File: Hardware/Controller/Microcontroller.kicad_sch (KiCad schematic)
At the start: 26 parts, among them J201 TagConnect_SWD, SW201 SW_Push, SW202 SW_Push, U201 W25Q64JVXGIQ, U202 RP2040, Y201 12M

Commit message: Changes and fixes
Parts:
- Y201: footprint Crystal:Crystal_SMD_Abracon_ABM3B-4Pin_5.0x3.2mm -> Crystal:Crystal_SMD_2520-4Pin_2.5x2.0mm; mouser 815-ABM3B1210B1UT -> 520-120-10-36Q-AEST
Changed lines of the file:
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@@
-	)
-	(symbol
-		(lib_id "Device:Crystal_GND24")
-		(at 38.1 152.4 90)
-		(unit 1)
-		(exclude_from_sim no)
-		(in_bom yes)
-		(on_board yes)
-		(dnp no)
-		(property "Reference" "Y201"
-			(at 38.1 142.24 90)
-			(effects
-				(font
-					(size 1.27 1.27)
-				)
-			)
-		)
-		(property "Value" "12M"
-			(at 38.1 144.78 90)
-			(effects
-				(font
-					(size 1.27 1.27)
-				)
-			)
-		)
-		(property "Footprint" "Crystal:Crystal_SMD_Abracon_ABM3B-4Pin_5.0x3.2mm"
-			(at 38.1 152.4 0)
-			(effects
-				(font
-					(size 1.27 1.27)
-				)
-				(hide yes)
-			)
-		)
-		(property "Datasheet" "https://eu.mouser.com/datasheet/2/3/abm3b-1774998.pdf"
-			(at 38.1 152.4 0)
-			(effects
-				(font
-					(size 1.27 1.27)
-				)
-				(hide yes)
-			)
-		)
-		(property "Description" ""
-			(at 38.1 152.4 0)
-			(effects
-				(font
-					(size 1.27 1.27)
-				)
-				(hide yes)
-			)
-		)
-		(property "mouser" "815-ABM3B1210B1UT"
-			(at 38.1 152.4 0)
-			(effects
-				(font
-					(size 1.27 1.27)
-				)
-				(hide yes)
-			)
-		)
-		(property "ETA" ""
-			(at 38.1 152.4 0)
-			(effects
-				(font
-					(size 1.27 1.27)
-				)
-				(hide yes)
-			)
-		)
-		(property "REASON" "ABM3B-12.000MHZ-10-B-1-U-T  is not sold at RS or elfa"
-			(at 38.1 152.4 0)
-			(effects
-				(font
-					(size 1.27 1.27)
-				)
-				(hide yes)
-			)
-		)
-		(property "RS-COMPONENTS" ""
-			(at 38.1 152.4 0)
-			(effects
-				(font
-					(size 1.27 1.27)
-				)
-				(hide yes)
-			)
-		)
-		(property "Footprint checked" "YES"
-			(at 38.1 152.4 0)
-			(effects
-				(font
-					(size 1.27 1.27)
-				)
-				(hide yes)
-			)
-		)
-		(pin "1"
-		)
-		(pin "2"
-		)
-		(pin "4"
-		)
-		(pin "3"
-		)
-		(instances
-			(project "Controller"
-				(path "/43ebced7-8538-4711-b1b5-1811dcfcbefa/a41632f7-ca6e-440e-a005-2089204e1c4a"
-					(reference "Y201")
-					(unit 1)
-				)
-			)
-		)
 	)
 	(symbol
@@
 					(unit 1)
 				)
+			)
+		)
+	)
+	(symbol
+		(lib_id "Device:Crystal_GND24")
+		(at 38.1 152.4 90)
+		(unit 1)
+		(exclude_from_sim no)
+		(in_bom yes)
+		(on_board yes)
+		(dnp no)
+		(property "Reference" "Y201"
+			(at 38.1 142.24 90)
+			(effects
+				(font
+					(size 1.27 1.27)
+				)
+			)
+		)
+		(property "Value" "12M"
+			(at 38.1 144.78 90)
+			(effects
+				(font
+					(size 1.27 1.27)
+				)
+			)
+		)
+		(property "Footprint" "Crystal:Crystal_SMD_2520-4Pin_2.5x2.0mm"
+			(at 38.1 152.4 0)
+			(effects
+				(font
+					(size 1.27 1.27)
+				)
+				(hide yes)
+			)
+		)
+		(property "Datasheet" "https://www.mouser.se/datasheet/2/122/ECX_2236Q-938171.pdf"
+			(at 38.1 152.4 0)
+			(effects
+				(font
+					(size 1.27 1.27)
+				)
+				(hide yes)
+			)
+		)
+		(property "Description" ""
+			(at 38.1 152.4 0)
+			(effects
+				(font
+					(size 1.27 1.27)
+				)
+				(hide yes)
+			)
+		)
+		(property "mouser" "520-120-10-36Q-AEST"
+			(at 38.1 152.4 0)
+			(effects
+				(font
+					(size 1.27 1.27)
+				)
+				(hide yes)
+			)
+		)
+		(property "ETA" ""
+			(at 38.1 152.4 0)
+			(effects
+				(font
+					(size 1.27 1.27)
+				)
+				(hide yes)
+			)
+		)
+		(property "REASON" "ABM3B-12.000MHZ-10-B-1-U-T  is not sold at RS or elfa"
+			(at 38.1 152.4 0)
+			(effects
+				(font
+					(size 1.27 1.27)
+				)
+				(hide yes)
+			)
+		)
+		(property "RS-COMPONENTS" ""
+			(at 38.1 152.4 0)
+			(effects
+				(font
+					(size 1.27 1.27)
+				)
+				(hide yes)
+			)
+		)
+		(property "Footprint checked" "YES"
+			(at 38.1 152.4 0)
+			(effects
+				(font
+					(size 1.27 1.27)
+				)
+				(hide yes)
+			)
+		)
+		(pin "1"
+		)
+		(pin "2"
+		)
+		(pin "4"
+		)
+		(pin "3"
+		)
+		(instances
+			(project "Controller"
+				(path "/43ebced7-8538-4711-b1b5-1811dcfcbefa/a41632f7-ca6e-440e-a005-2089204e1c4a"
+					(reference "Y201")
+					(unit 1)
+				)

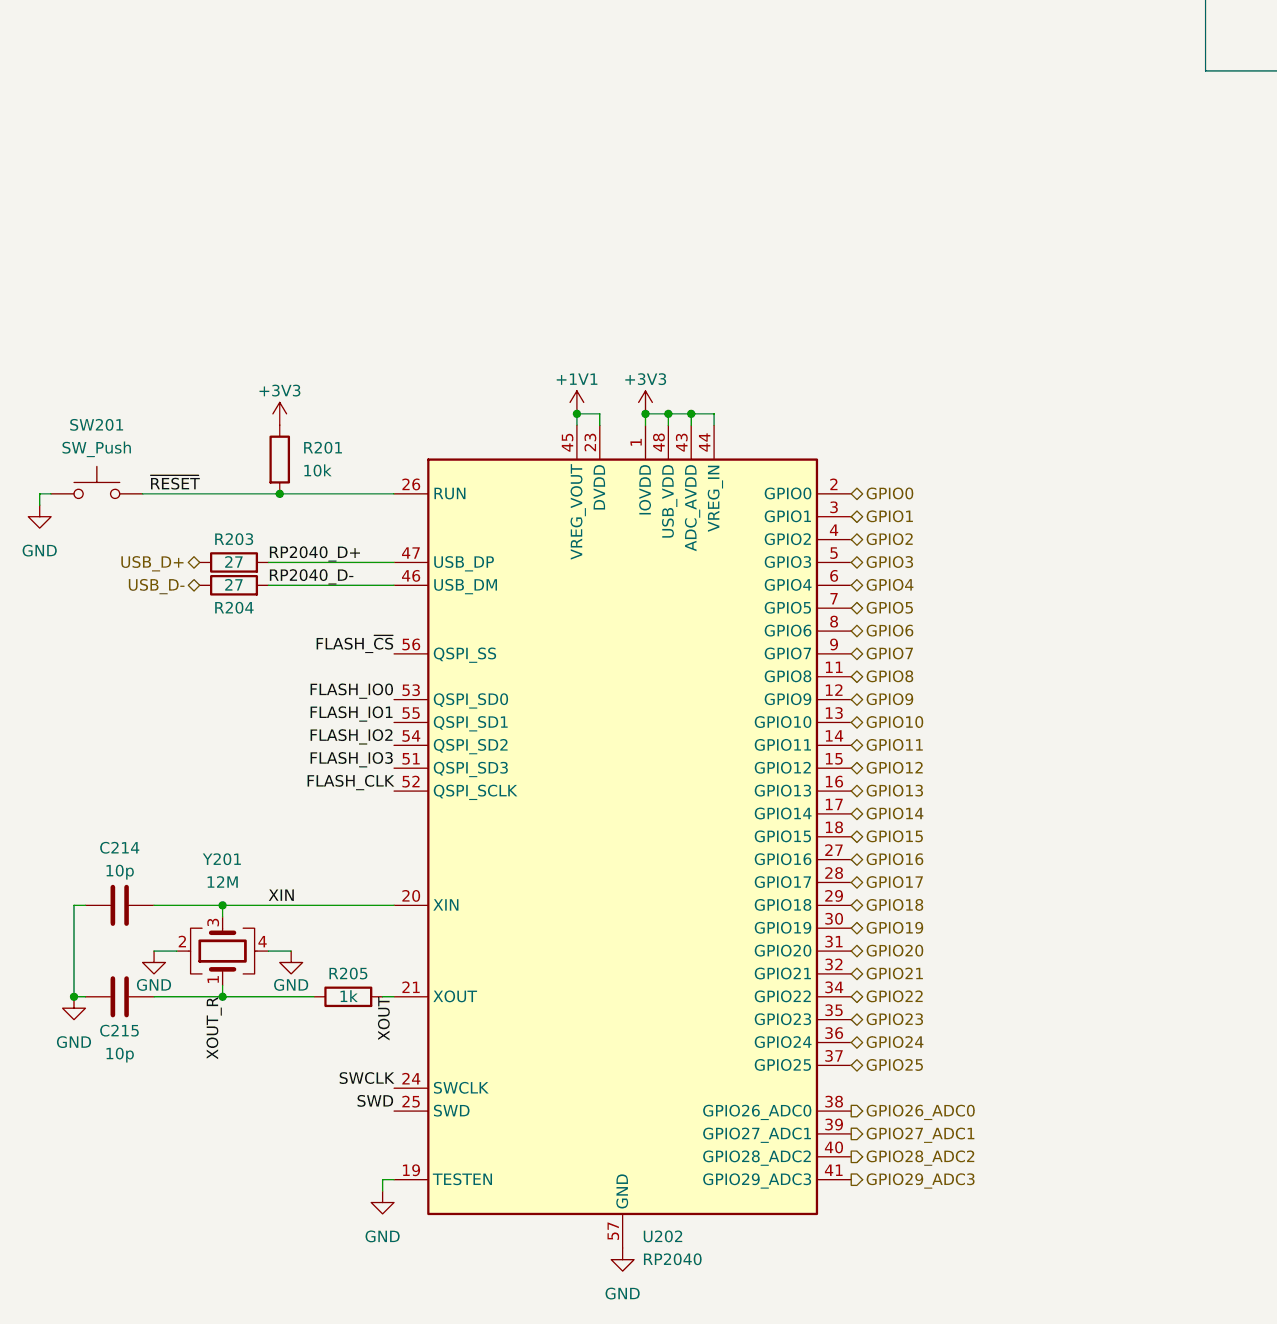
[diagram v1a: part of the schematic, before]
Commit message: final fixes (hopefully) (GONE WRONG?!) (real)
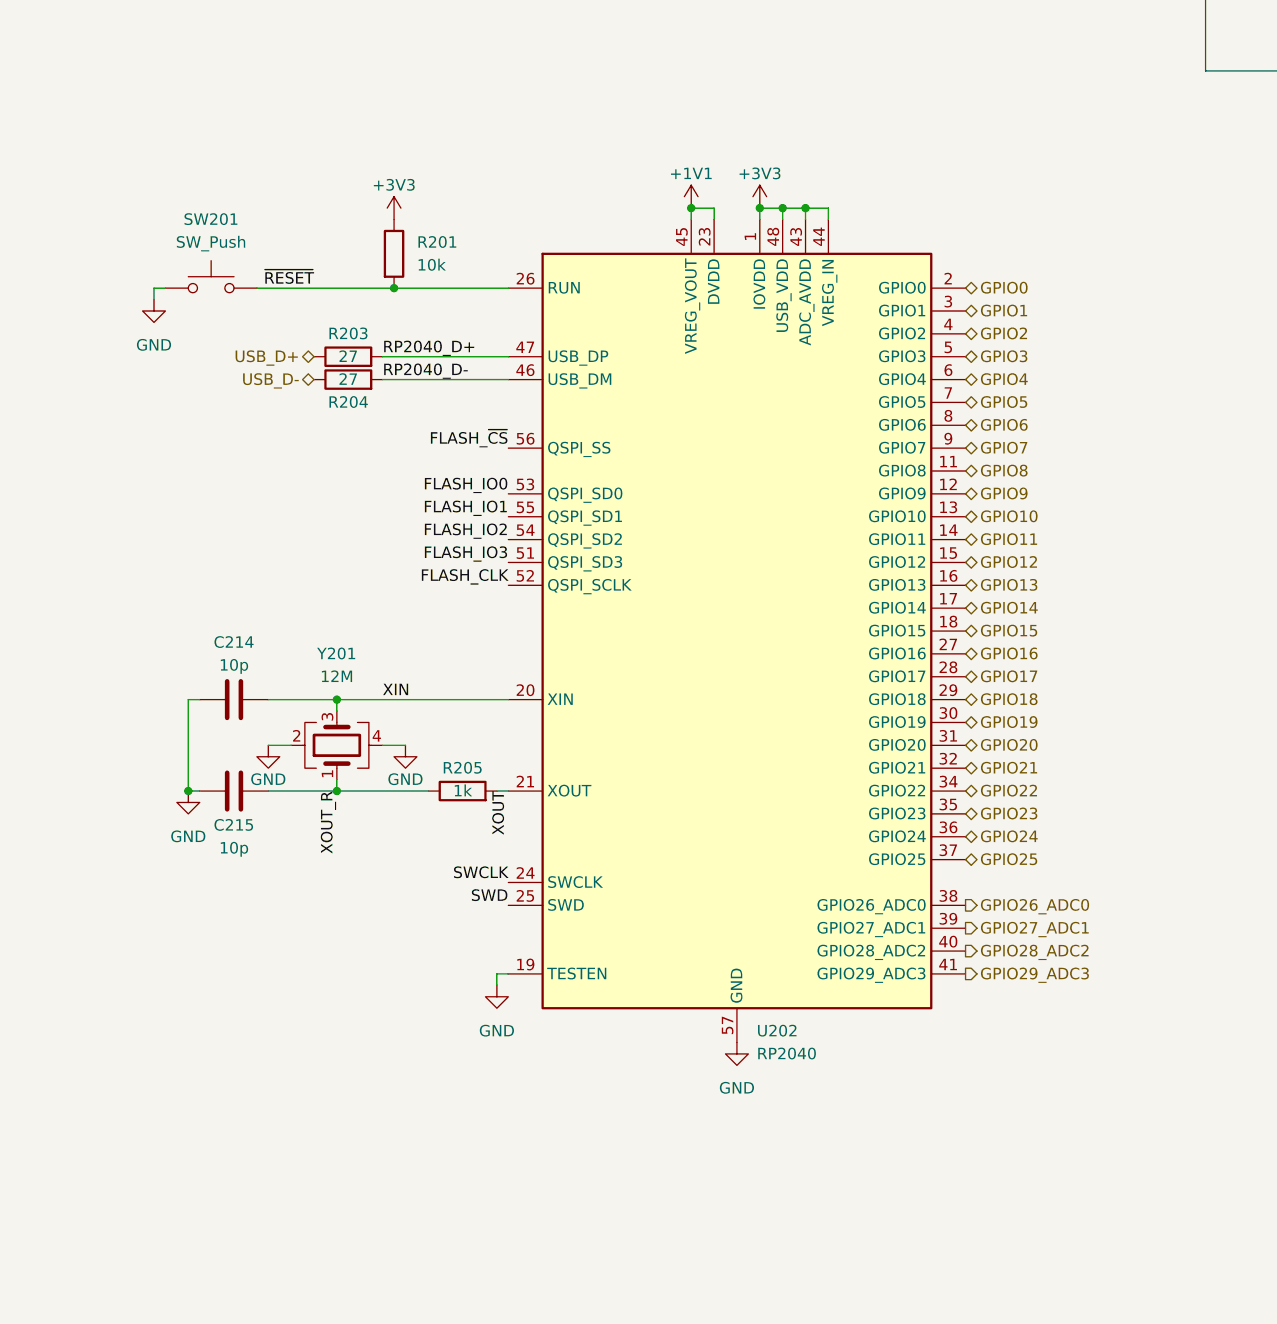
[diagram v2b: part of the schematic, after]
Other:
- title: (none) -> RP2040 Microcontroller and support components
- moved on the sheet: C214, C215, R201, R203, R204, R205, SW201, U202, Y201
